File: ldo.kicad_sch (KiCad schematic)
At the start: 8 parts, among them Q6 NMOS, U19 OPA705PA

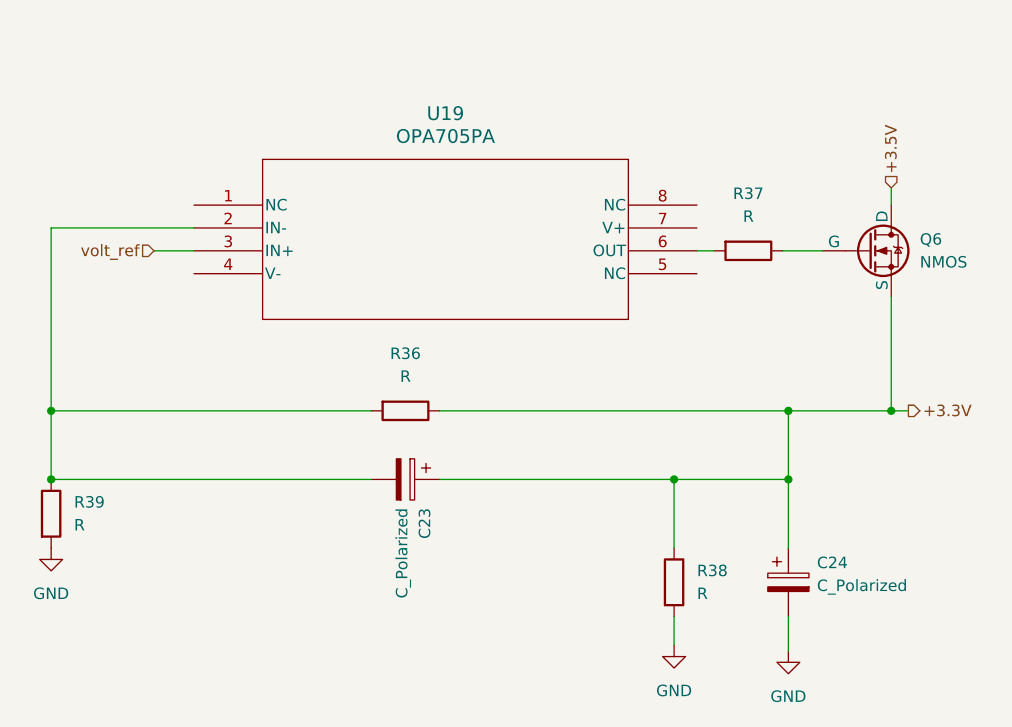
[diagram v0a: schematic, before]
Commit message: schematic cleanup
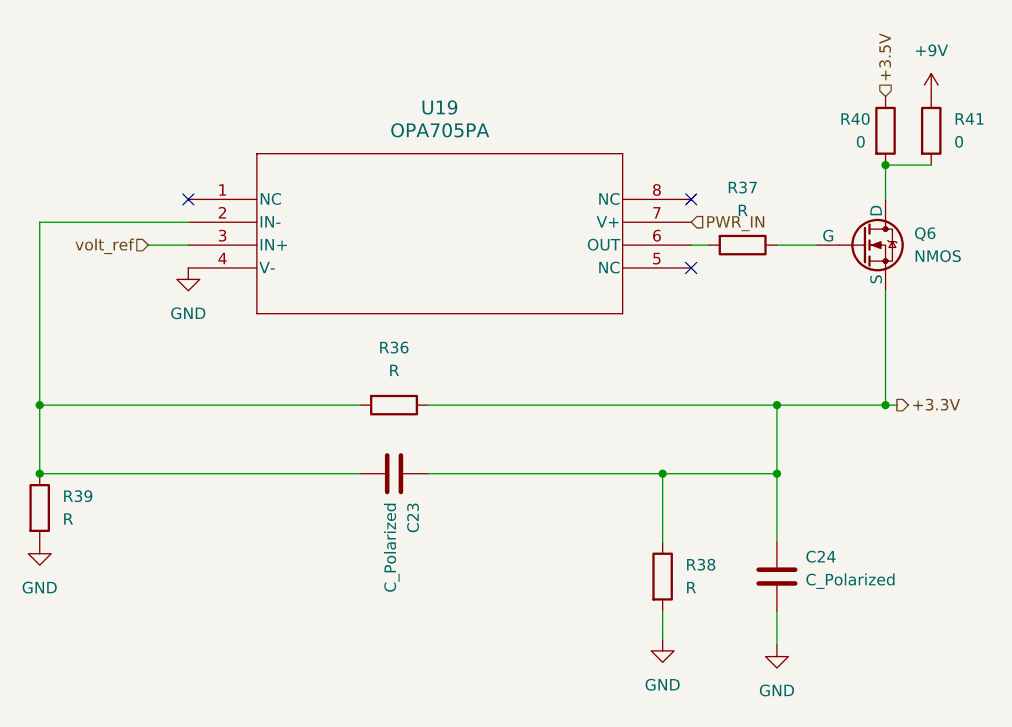
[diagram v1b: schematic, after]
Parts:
- added R40, R41: 0, Resistor_SMD:R_0805_2012Metric, symbol Device:R
- C23, C24: footprint (none) -> Capacitor_SMD:C_0805_2012Metric; symbol Device:C_Polarized -> Device:C
- R36, R37, R38, R39: footprint (none) -> Resistor_SMD:R_0805_2012Metric
- U19: footprint footprints10:P8 -> footprints:P8
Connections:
- net +3.5V: now also R40.1; no longer Q6.2 (D)
- net GND: now also U19.4 (V-)
- net PWR_IN: now reaches U19.7 (V+)
- new net: Q6.2 (D), R40.2, R41.2
- new net +9V: R41.1
- no-connect marks 0 -> 3
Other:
- moved on the sheet: Q6, R36, R37, R38, R39, U19
